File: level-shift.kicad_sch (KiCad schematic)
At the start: 3 parts, among them Q2 2N7002K

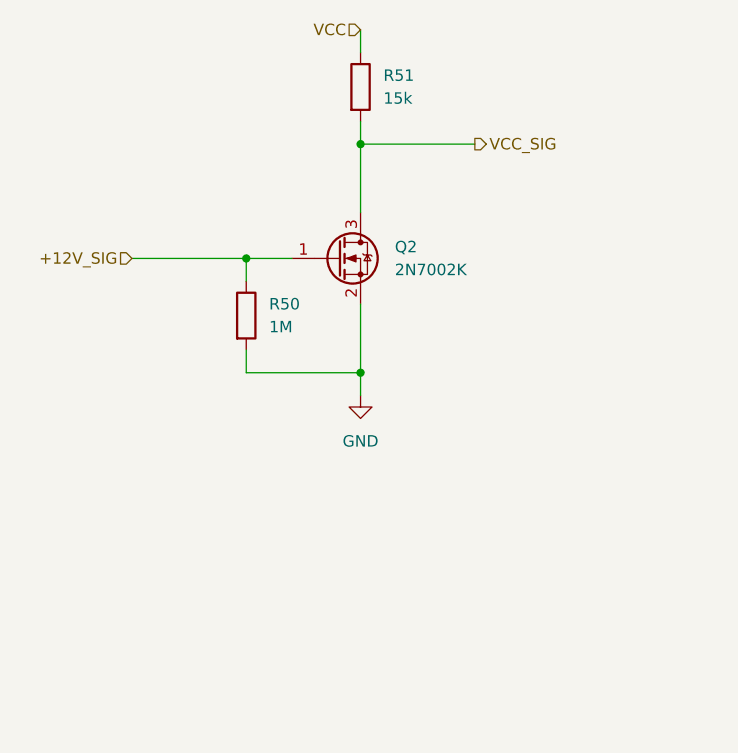
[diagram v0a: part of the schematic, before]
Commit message: シャットダウン検知をMOSFETから分圧回路に変更、リファレンス指定子"IC?"を"U?"に変更
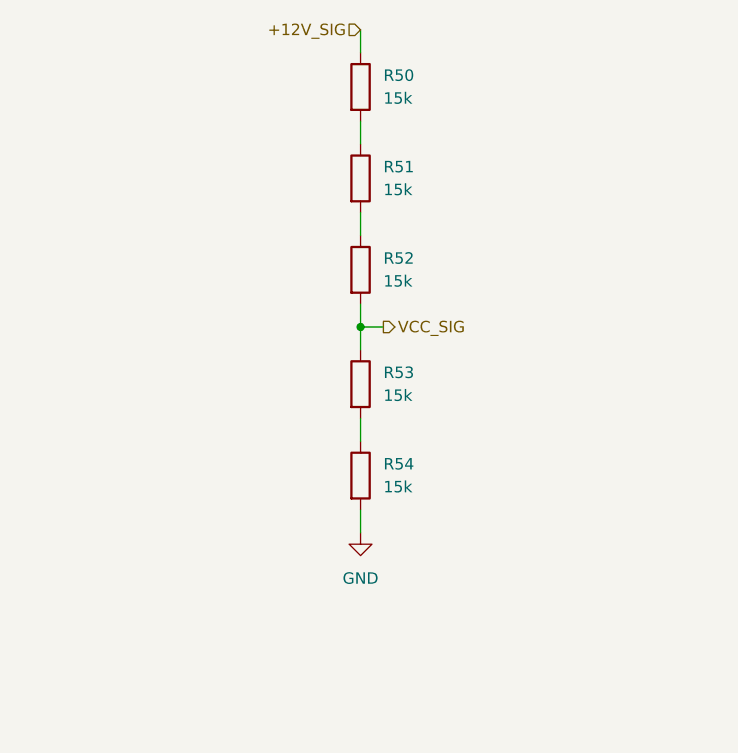
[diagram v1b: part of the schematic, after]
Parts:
- removed Q2: 2N7002K, Package_TO_SOT_SMD:SOT-23, symbol Transistor_FET:2N7002K
- added R52, R53, R54: 15k, Resistor_SMD:R_0603_1608Metric, symbol Device:R
- R50: value 1M -> 15k
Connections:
- net GND: now also R54.2; no longer R50.2
- net VCC_SIG: now also R52.2, R53.1; no longer R51.2
- net VCC: no longer names the net of R51.1
- net VCC: now also R50.2
- new net: R53.2, R54.1
- new net: R51.2, R52.1
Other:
- moved on the sheet: R50, R51
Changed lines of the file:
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@@
 (kicad_sch (version 20230121) (generator eeschema)
   (paper "A4")
-  (junction (at 127 101.6) (diameter 0) (color 0 0 0 0)
+  (junction (at 127 96.52) (diameter 0) (color 0 0 0 0)
   )
-  (junction (at 127 76.2) (diameter 0) (color 0 0 0 0)
+  (wire (pts (xy 127 63.5) (xy 127 66.04))
+    (stroke (width 0) (type default))
   )
-  (junction (at 114.3 88.9) (diameter 0) (color 0 0 0 0)
+  (wire (pts (xy 127 96.52) (xy 127 99.06))
+    (stroke (width 0) (type default))
   )
-  (wire (pts (xy 127 76.2) (xy 127 83.82))
+  (wire (pts (xy 127 96.52) (xy 129.54 96.52))
+    (stroke (width 0) (type default))
+  )
+  (wire (pts (xy 127 106.68) (xy 127 109.22))
+    (stroke (width 0) (type default))
+  )
+  (wire (pts (xy 127 93.98) (xy 127 96.52))
+    (stroke (width 0) (type default))
+  )
+  (wire (pts (xy 127 116.84) (xy 127 119.38))
     (stroke (width 0) (type default))
   )
@@
     (stroke (width 0) (type default))
   )
-  (wire (pts (xy 127 93.98) (xy 127 101.6))
-    (stroke (width 0) (type default))
-  )
-  (wire (pts (xy 114.3 88.9) (xy 114.3 91.44))
-    (stroke (width 0) (type default))
-  )
-  (wire (pts (xy 127 63.5) (xy 127 66.04))
-    (stroke (width 0) (type default))
-  )
-  (wire (pts (xy 127 76.2) (xy 139.7 76.2))
-    (stroke (width 0) (type default))
-  )
-  (wire (pts (xy 127 101.6) (xy 127 104.14))
-    (stroke (width 0) (type default))
-  )
-  (wire (pts (xy 114.3 88.9) (xy 119.38 88.9))
-    (stroke (width 0) (type default))
-  )
-  (wire (pts (xy 101.6 88.9) (xy 114.3 88.9))
-    (stroke (width 0) (type default))
-  )
-  (wire (pts (xy 114.3 101.6) (xy 127 101.6))
-    (stroke (width 0) (type default))
-  )
-  (wire (pts (xy 114.3 99.06) (xy 114.3 101.6))
+  (wire (pts (xy 127 83.82) (xy 127 86.36))
     (stroke (width 0) (type default))
   )
@@
     (effects (font (size 5.08 5.08)) (justify left bottom))
   )
-  (hierarchical_label "VCC_SIG" (shape output) (at 139.7 76.2 0) (fields_autoplaced)
+  (hierarchical_label "VCC_SIG" (shape output) (at 129.54 96.52 0) (fields_autoplaced)
     (effects (font (size 1.27 1.27)) (justify left))
   )
-  (hierarchical_label "VCC" (shape input) (at 127 63.5 180) (fields_autoplaced)
+  (hierarchical_label "+12V_SIG" (shape input) (at 127 63.5 180) (fields_autoplaced)
     (effects (font (size 1.27 1.27)) (justify right))
   )
-  (hierarchical_label "+12V_SIG" (shape input) (at 101.6 88.9 180) (fields_autoplaced)
-    (effects (font (size 1.27 1.27)) (justify right))
-  )
-  (symbol (lib_id "Transistor_FET:2N7002K") (at 124.46 88.9 0) (unit 1)
+  (symbol (lib_id "Device:R") (at 127 102.87 0) (unit 1)
     (in_bom yes) (on_board yes) (dnp no) (fields_autoplaced)
-    (property "Reference" "Q2" (at 130.81 87.63 0)
+    (property "Reference" "R53" (at 129.54 101.6 0)
       (effects (font (size 1.27 1.27)) (justify left))
     )
-    (property "Value" "2N7002K" (at 130.81 90.17 0)
+    (property "Value" "15k" (at 129.54 104.14 0)
       (effects (font (size 1.27 1.27)) (justify left))
     )
-    (property "Footprint" "Package_TO_SOT_SMD:SOT-23" (at 129.54 90.805 0)
-      (effects (font (size 1.27 1.27) italic) (justify left) hide)
+    (property "Footprint" "Resistor_SMD:R_0603_1608Metric" (at 125.222 102.87 90)
+      (effects (font (size 1.27 1.27)) hide)
     )
-    (property "Datasheet" "https://www.diodes.com/assets/Datasheets/ds30896.pdf" (at 124.46 88.9 0)
-      (effects (font (size 1.27 1.27)) (justify left) hide)
+    (property "Datasheet" "~" (at 127 102.87 0)
+      (effects (font (size 1.27 1.27)) hide)
     )
-    (property "発注先" "秋月電子" (at 124.46 88.9 0)
+    (property "発注先" "Digi-Key" (at 127 102.87 0)
       (effects (font (size 1.27 1.27)) hide)
     )
     (pin "1")
     (pin "2")
-    (pin "3")
     (instances
       (project "main-ECU-board"
         (path "/10edd9b6-c7a8-40f4-bfe3-c9724324d30f/aaf3b5fe-1b86-4630-ab8c-ff326b8bda0a"
-          (reference "Q2") (unit 1)
+          (reference "R53") (unit 1)
+        )
+      )
+    )
+  )
+  (symbol (lib_id "Device:R") (at 127 113.03 0) (unit 1)
+    (in_bom yes) (on_board yes) (dnp no) (fields_autoplaced)
+    (property "Reference" "R54" (at 129.54 111.76 0)
+      (effects (font (size 1.27 1.27)) (justify left))
+    )
+    (property "Value" "15k" (at 129.54 114.3 0)
+      (effects (font (size 1.27 1.27)) (justify left))
+    )
+    (property "Footprint" "Resistor_SMD:R_0603_1608Metric" (at 125.222 113.03 90)
+      (effects (font (size 1.27 1.27)) hide)
+    )
+    (property "Datasheet" "~" (at 127 113.03 0)
+      (effects (font (size 1.27 1.27)) hide)
+    )
+    (property "発注先" "Digi-Key" (at 127 113.03 0)
+      (effects (font (size 1.27 1.27)) hide)
+    )
+    (pin "1")
+    (pin "2")
+    (instances
+      (project "main-ECU-board"
+        (path "/10edd9b6-c7a8-40f4-bfe3-c9724324d30f/aaf3b5fe-1b86-4630-ab8c-ff326b8bda0a"
+          (reference "R54") (unit 1)
+        )
+      )
+    )
+  )
+  (symbol (lib_id "Device:R") (at 127 80.01 0) (unit 1)
+    (in_bom yes) (on_board yes) (dnp no) (fields_autoplaced)
+    (property "Reference" "R51" (at 129.54 78.74 0)
+      (effects (font (size 1.27 1.27)) (justify left))
+    )
+    (property "Value" "15k" (at 129.54 81.28 0)
+      (effects (font (size 1.27 1.27)) (justify left))
+    )
+    (property "Footprint" "Resistor_SMD:R_0603_1608Metric" (at 125.222 80.01 90)
+      (effects (font (size 1.27 1.27)) hide)
+    )
+    (property "Datasheet" "~" (at 127 80.01 0)
+      (effects (font (size 1.27 1.27)) hide)
+    )
+    (property "発注先" "Digi-Key" (at 127 80.01 0)
+      (effects (font (size 1.27 1.27)) hide)
+    )
+    (pin "1")
+    (pin "2")
+    (instances
+      (project "main-ECU-board"
+        (path "/10edd9b6-c7a8-40f4-bfe3-c9724324d30f/aaf3b5fe-1b86-4630-ab8c-ff326b8bda0a"
+          (reference "R51") (unit 1)
+        )
+      )
+    )
+  )
+  (symbol (lib_id "Device:R") (at 127 90.17 0) (unit 1)
+    (in_bom yes) (on_board yes) (dnp no) (fields_autoplaced)
+    (property "Reference" "R52" (at 129.54 88.9 0)
+      (effects (font (size 1.27 1.27)) (justify left))
+    )
+    (property "Value" "15k" (at 129.54 91.44 0)
+      (effects (font (size 1.27 1.27)) (justify left))
+    )
+    (property "Footprint" "Resistor_SMD:R_0603_1608Metric" (at 125.222 90.17 90)
+      (effects (font (size 1.27 1.27)) hide)
+    )
+    (property "Datasheet" "~" (at 127 90.17 0)
+      (effects (font (size 1.27 1.27)) hide)
+    )
+    (property "発注先" "Digi-Key" (at 127 90.17 0)
+      (effects (font (size 1.27 1.27)) hide)
+    )
+    (pin "1")
+    (pin "2")
+    (instances
+      (project "main-ECU-board"
+        (path "/10edd9b6-c7a8-40f4-bfe3-c9724324d30f/aaf3b5fe-1b86-4630-ab8c-ff326b8bda0a"
+          (reference "R52") (unit 1)
         )
       )
@@
   (symbol (lib_id "Device:R") (at 127 69.85 0) (unit 1)
     (in_bom yes) (on_board yes) (dnp no) (fields_autoplaced)
-    (property "Reference" "R51" (at 129.54 68.58 0)
+    (property "Reference" "R50" (at 129.54 68.58 0)
       (effects (font (size 1.27 1.27)) (justify left))
     )
@@
       (project "main-ECU-board"
         (path "/10edd9b6-c7a8-40f4-bfe3-c9724324d30f/aaf3b5fe-1b86-4630-ab8c-ff326b8bda0a"
-          (reference "R51") (unit 1)
-        )
-      )
-    )
-  )
-  (symbol (lib_id "Device:R") (at 114.3 95.25 0) (unit 1)
-    (in_bom yes) (on_board yes) (dnp no) (fields_autoplaced)
-    (property "Reference" "R50" (at 116.84 93.98 0)
-      (effects (font (size 1.27 1.27)) (justify left))
-    )
-    (property "Value" "1M" (at 116.84 96.52 0)
-      (effects (font (size 1.27 1.27)) (justify left))
-    )
-    (property "Footprint" "Resistor_SMD:R_0603_1608Metric" (at 112.522 95.25 90)
-      (effects (font (size 1.27 1.27)) hide)
-    )
-    (property "Datasheet" "~" (at 114.3 95.25 0)
-      (effects (font (size 1.27 1.27)) hide)
-    )
-    (property "発注先" "Digi-Key" (at 114.3 95.25 0)
-      (effects (font (size 1.27 1.27)) hide)
-    )
-    (pin "1")
-    (pin "2")
-    (instances
-      (project "main-ECU-board"
-        (path "/10edd9b6-c7a8-40f4-bfe3-c9724324d30f/aaf3b5fe-1b86-4630-ab8c-ff326b8bda0a"
           (reference "R50") (unit 1)
         )
@@
     )
   )
-  (symbol (lib_id "power:GND") (at 127 104.14 0) (unit 1)
+  (symbol (lib_id "power:GND") (at 127 119.38 0) (unit 1)
     (in_bom yes) (on_board yes) (dnp no) (fields_autoplaced)
-    (property "Reference" "#PWR086" (at 127 110.49 0)
+    (property "Reference" "#PWR086" (at 127 125.73 0)
       (effects (font (size 1.27 1.27)) hide)
     )
-    (property "Value" "GND" (at 127 109.22 0)
+    (property "Value" "GND" (at 127 124.46 0)
       (effects (font (size 1.27 1.27)))
     )
-    (property "Footprint" "" (at 127 104.14 0)
+    (property "Footprint" "" (at 127 119.38 0)
       (effects (font (size 1.27 1.27)) hide)
     )
-    (property "Datasheet" "" (at 127 104.14 0)
+    (property "Datasheet" "" (at 127 119.38 0)
       (effects (font (size 1.27 1.27)) hide)
     )
